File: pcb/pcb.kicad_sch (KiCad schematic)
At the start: 46 parts, among them J1 Conn_02x08_Top_Bottom, J2 Conn_02x08_Top_Bottom, SW1 CherryMX_LED, SW2 CherryMX_LED, SW3 1241.1100.7095, SW4 SW_SPST, U1 ICM7211AMIPL, U2 ICM7211AMIPL, U3 ATTINY84A, U4 NL37WZ14USG, U5 SN74AHC138DR, U6 MAX5035BUSA+, U6 SN74F02D, U7 TC7WZ32FK_LJCT, Y1 Crystal

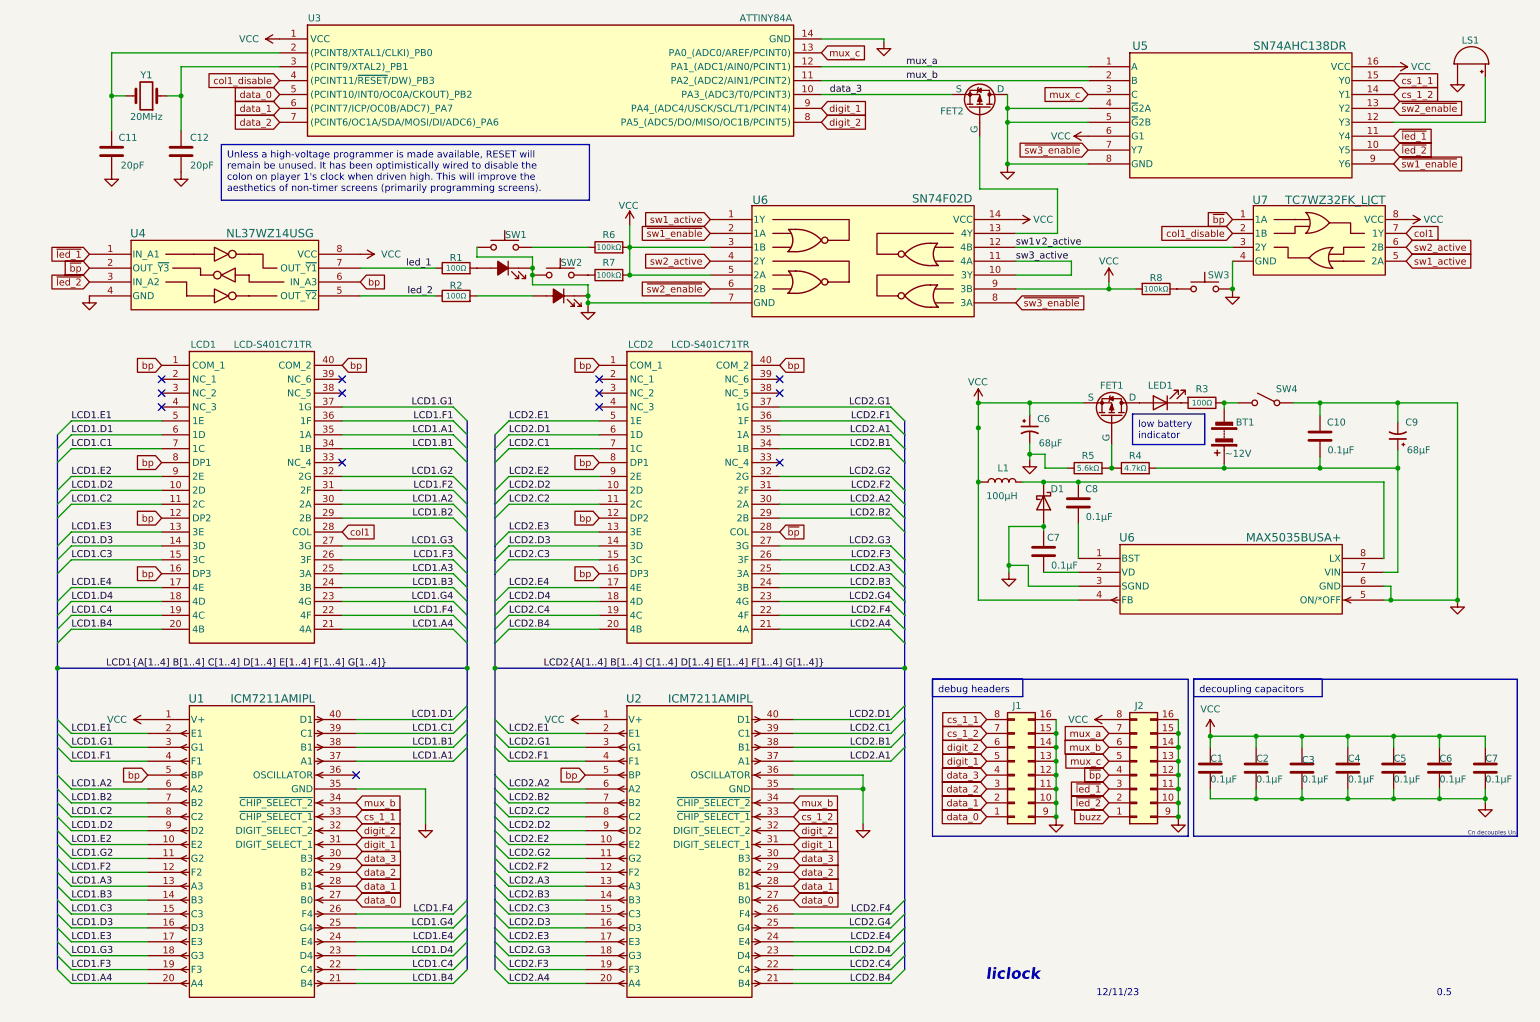
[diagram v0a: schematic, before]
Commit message: initialize pcb design
Signed-off-by: Michael Darr <michael.e.darr@gmail.com>
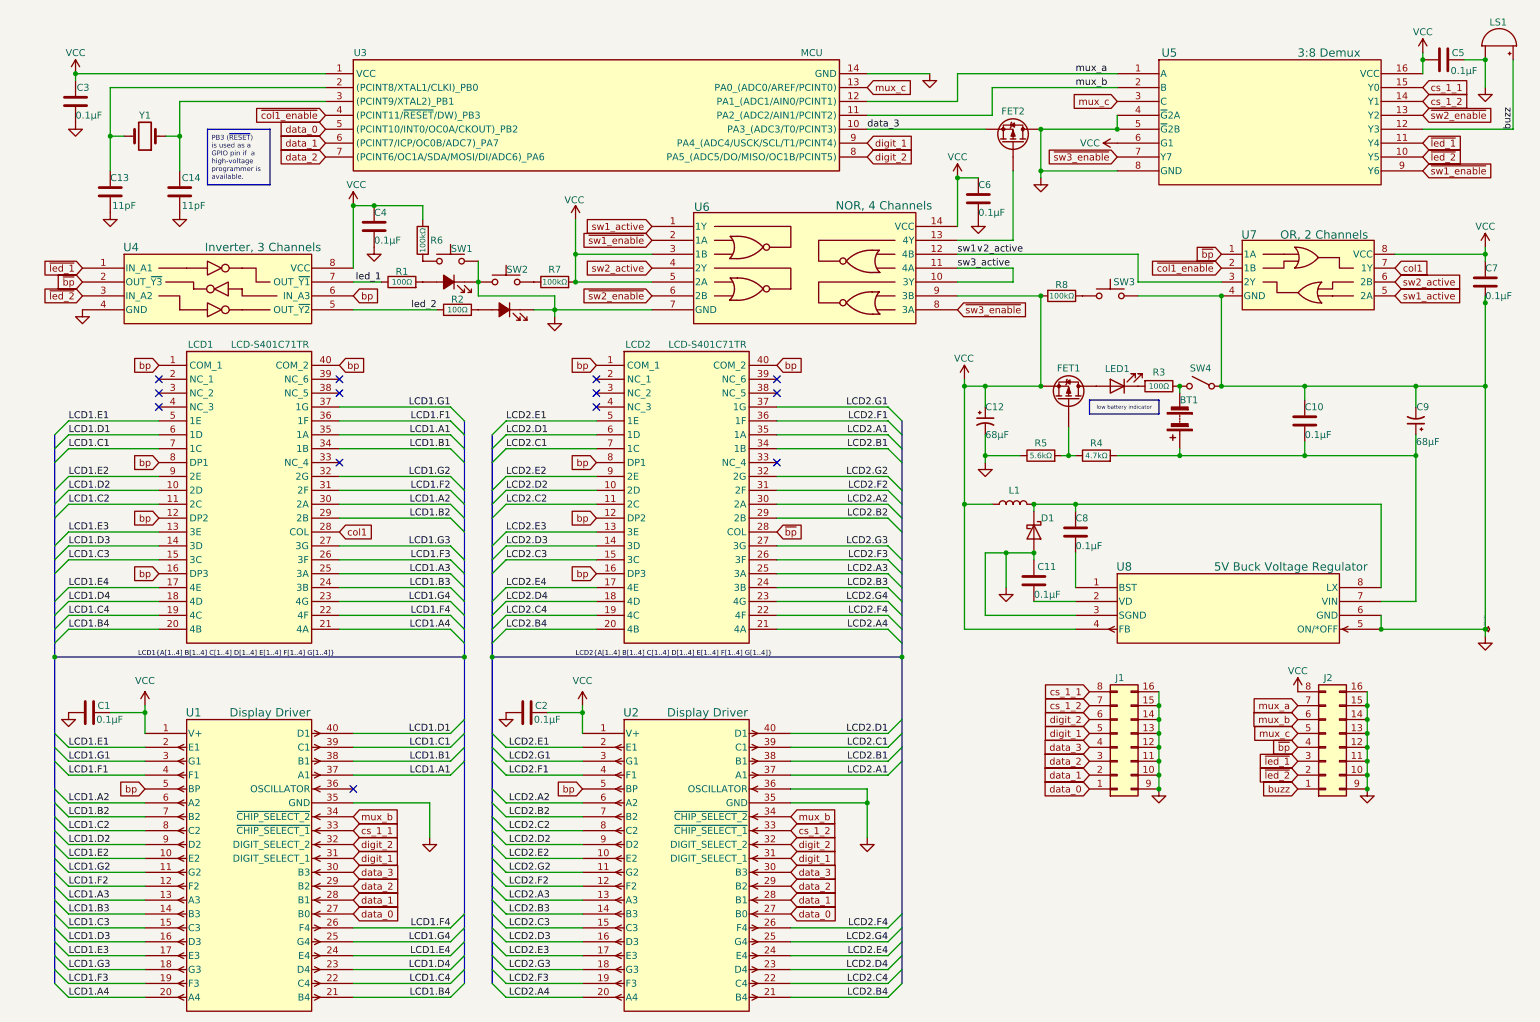
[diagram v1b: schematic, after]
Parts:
- BT1: value Battery -> ~9V; footprint (none) -> Connector_Wire:SolderWire-0.15sqmm_1x02_P4mm_D0.5mm_OD1.5mm; Capacity ~5Ah -> (none); Cells 6 * AAA -> (none); Manufacturer_Name (none) -> Memory Protection Devices, Inc; Notes (none) -> 6 AAA batteries, ~9Ah; PN (none) -> BH26AAAW; Volatage ~12V -> (none)
- C1, C2, C3, C4, C5, C6, C7: footprint (none) -> chess_clock:RDER71H104K0M1H03A; Capacitance (none) -> 0.1µF; Manufacturer_Name (none) -> Murata; Notes (none) -> Ceramic Capacitor; PN (none) -> RDER71H104K0M1H03A
- C10: value C -> 0.1µF; footprint (none) -> chess_clock:RDER71H104K0M1H03A; Manufacturer_Name (none) -> Murata; Notes datasheet, pg 12: "Use a 1µF or greater value ceramic capac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 -> Ceramic Capacitor; PN (none) -> RDER71H104K0M1H03A; Type ceramic -> (none)
- C11: renamed from C7; value C -> 0.1µF; footprint (none) -> chess_clock:RDER71H104K0M1H03A; Manufacturer_Name (none) -> Murata; Notes (none) -> Ceramic Capacitor; PN (none) -> RDER71H104K0M1H03A; Spec page 9: "Bypass VD to GND with a 0.1µF ceramic capacitor." -> (none); Type ceramic -> (none)
- C12: renamed from C6; value C_Polarized_Small_US -> 68µF; footprint (none) -> chess_clock:TPSD686K010R0100; Manufacturer_Name (none) -> KYOCERA AVX; Notes (none) -> Polarized Capacitor; PN (none) -> TPSD686K010R0100
- C13: renamed from C11; value C -> 11pF; footprint (none) -> chess_clock:GJM1555C1H110FB01D; Capacitance 20pF -> 11pF; Manufacturer_Name (none) -> Murata; Notes (none) -> Ceramic Capacitor; PN (none) -> GJM1555C1H110FB01D
- C14: renamed from C12; value C -> 11pF; footprint (none) -> chess_clock:GJM1555C1H110FB01D; Capacitance 20pF -> 11pF; Manufacturer_Name (none) -> Murata; Notes (none) -> Ceramic Capacitor; PN (none) -> GJM1555C1H110FB01D
- C8: value C -> 0.1µF; footprint (none) -> chess_clock:RDER71H104K0M1H03A; Manufacturer_Name (none) -> Murata; Notes (none) -> Ceramic Capacitor; PN (none) -> RDER71H104K0M1H03A; Spec pg. 9: "Connect a 0.1µF ceramic capacitor from BST to LX." -> (none); Type ceramic -> (none)
- C9: value C_Polarized_Small_US -> 68µF; footprint (none) -> chess_clock:TPSD686K010R0100; Manufacturer_Name (none) -> KYOCERA AVX; Notes TODO => calculate precise capacitance (pg. 11/12) -> Polarized Capacitor; PN (none) -> TPSD686K010R0100
- D1: value D_Schottky -> Schottky Diode; footprint (none) -> chess_clock:B240AE-13; Manufacturer_Name (none) -> Diodes Inc.; Notes (none) -> Schottky Diode | page 11, table 1, 7.5 to 36; PN (none) -> B240AE-13; PN - Central Semiconductor B240 -> (none); PN - Diodes, Inc B240A -> (none); PN - IR 15MQ040N -> (none); PN - ON Semiconductor MBRS240, MBRS1540 -> (none); Spec page 11, table 1, 7.5 to 36 (PN recommendations reproduced 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 -> (none)
- FET1, FET2: value XP9561GI -> PMOS; footprint (none) -> Package_TO_SOT_THT:TO-220-3_Vertical; Manufacturer_Name (none) -> Yageo; PN (none) -> XP9561GI
- J1, J2: value Conn_02x08_Top_Bottom -> Dubugging Headers; footprint (none) -> chess_clock:10129381-916001BLF; Manufacturer_Name (none) -> Amphenol; PN (none) -> 10129381-916001BLF
- L1: value L -> 100μH; footprint (none) -> chess_clock:DO5022P-104MLD; Inductance 100μH -> (none); Manufacturer_Name (none) -> Coilcraft; PN (none) -> DO5022P-104MLD
- LCD1, LCD2: footprint DIP4000W30P254L6985H218Q40N -> chess_clock:LCD-S401C71TR; Arrow Part Number LCD-S401C71TR -> (none); Arrow Price/Stock https://www.arrow.com/en/products/lcd-s401c71tr/lumex -> (none); Height 2.18 -> (none); Manufacturer_Part_Number LCD-S401C71TR -> (none); Mouser Part Number 696-LCD-S401C71TR -> (none); Mouser Price/Stock https://www.mouser.co.uk/ProductDetail/Lumex/LCD-S401C71TR?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 -> (none); PN (none) -> LCD-S401C71TR
- LED1: value 151033RS03000 -> Red low battery Indicator; footprint (none) -> LED_THT:LED_D3.0mm_Clear; Manufacturer_Name (none) -> Wurth Elektronik; PN (none) -> 151033RS03000
- LS1: footprint (none) -> chess_clock:CT-1205H-SMT; Manufacturer_Name (none) -> CUI Devices; PN (none) -> CT-1205H-SMT-TR
- R1, R2, R3: footprint (none) -> Resistor_THT:R_Axial_DIN0204_L3.6mm_D1.6mm_P2.54mm_Vertical; Manufacturer_Name (none) -> TE connectivity; PN (none) -> ROX1SJ100R
- R4: footprint (none) -> Resistor_THT:R_Axial_DIN0204_L3.6mm_D1.6mm_P2.54mm_Vertical; Manufacturer_Name (none) -> TE connectivity; PN (none) -> CFR16J4K7
- R5: footprint (none) -> Resistor_THT:R_Axial_DIN0204_L3.6mm_D1.6mm_P2.54mm_Vertical; Manufacturer_Name (none) -> TE connectivity; PN (none) -> CFR50J5K6
- R6, R7, R8: footprint (none) -> Resistor_THT:R_Axial_DIN0204_L3.6mm_D1.6mm_P2.54mm_Vertical; Manufacturer_Name (none) -> TE connectivity; PN (none) -> ROX1SJ100K
- SW1, SW2: value CherryMX_LED -> Cherry MX Grey Switch w/ Green LED; footprint (none) -> chess_clock:MX_LED; Manufacturer_Name (none) -> Cherry; Notes (none) -> LED PN: INL-3AG30 [datasheet](https://www.inolux-corp.com/d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; PN (none) -> MX1A-D1NA
- SW3: footprint (none) -> chess_clock:MCS 18 Front; Manufacturer_Name (none) -> Schurter; PN (none) -> 1241.1100.7095
- SW4: footprint (none) -> chess_clock:CWSA11AAN1H; Manufacturer_Name (none) -> NKK Switches; PN (none) -> CWSA11AAN1H
- U1, U2: value ICM7211AMIPL -> Display Driver; footprint 21-0044B_40_MXM -> chess_clock:ICM7211AMIPL; Manufacturer_Name (none) -> Maxim; PN (none) -> ICM7211AMIPL
- U3: value ATTINY84A -> MCU; footprint DIP794W56P254L1918H533Q14N -> chess_clock:ATtiny84a; Height 5.334 -> (none); Manufacturer_Part_Number ATTINY48A-PU -> (none); PN (none) -> ATTINY84A
- U4: value NL37WZ14USG -> Inverter, 3 Channels; footprint US8_2P40X2P10_ONS -> chess_clock:NL37WZ14USG; Manufacturer_Name (none) -> Onsemi; PN (none) -> NL37WZ14USG
- U5: value SN74AHC138DR -> 3:8 Demux; footprint D16 -> chess_clock:SN74AHC138DR; Manufacturer_Name (none) -> Texas Instruments; PN (none) -> SN74AHC138DR
- U6: value SN74F02D -> NOR, 4 Channels; footprint D14 -> chess_clock:SN74F02D; Manufacturer_Name (none) -> Texas Instruments; PN (none) -> SN74F02D
- U7: value TC7WZ32FK_LJCT -> OR, 2 Channels; footprint US8_TOS -> chess_clock:TC7WZ32FK_LJCT; Manufacturer_Name (none) -> Toshiba; PN (none) -> TC7WZ32FK
- U8: renamed from U6; value MAX5035BUSA+ -> 5V Buck Voltage Regulator; footprint 21-0041B_8_MXM -> chess_clock:MAX5035BUSA+; Manufacturer_Name (none) -> Maxim; PN (none) -> MAX5035BUSA+
- Y1: value Crystal -> 20MHz Crystal; footprint (none) -> chess_clock:ECS_200_18_4X_CKM; Frequency 20MHz -> (none); Manufacturer_Name (none) -> ECS Inc; PN (none) -> ECS-200-18-4X-CKM
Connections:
- net GND: now also C1.1, C2.1, C3.1, SW1.1; no longer C1.2, C2.2, C3.2, SW1.2
- net VCC: now also C1.2, C2.2, C3.2; no longer C1.1, C2.1, C3.1
- net buzz: now also LS1.1 (-), U5.12 (Y3)
- net at R6.1: now also SW1.2; no longer SW1.1
- net col1_disable renamed ~{col1_enable}
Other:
- note removed: "0.5"
- note removed: "12/11/23"
- note removed: "Cn decouples Un"
- note removed: "liclock"
- company: (none) -> Alset
- title: (none) -> Liclock
- moved on the sheet: BT1, C1, C10, C11, C12, C13, C14, C2, C3, C4, C5, C6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
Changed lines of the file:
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@@
 (kicad_sch (version 20230121) (generator eeschema)
   (paper "A4")
+  (title_block
+    (title "Liclock")
+    (date "2023-12-12")
+    (rev "0,6")
+    (company "Alset")
+  )
